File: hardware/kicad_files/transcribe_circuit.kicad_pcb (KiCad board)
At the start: 2 copper layers, 100 x 45 mm, 25 parts, among them J1 europower, J2 RS232_SERIAL, J3 RS232_DSUB, J4 MIDI_IN_TRS, J5 MIDI_IN_DIN, J6 MIDI_OUT_TRS, J7 MIDI_OUT_DIN, J8 Conn_01x06, U1 ProMicro, U2 MAX232, U3 6N137, U4 4069, U5 usbHostMini, U6 L78L33_TO92

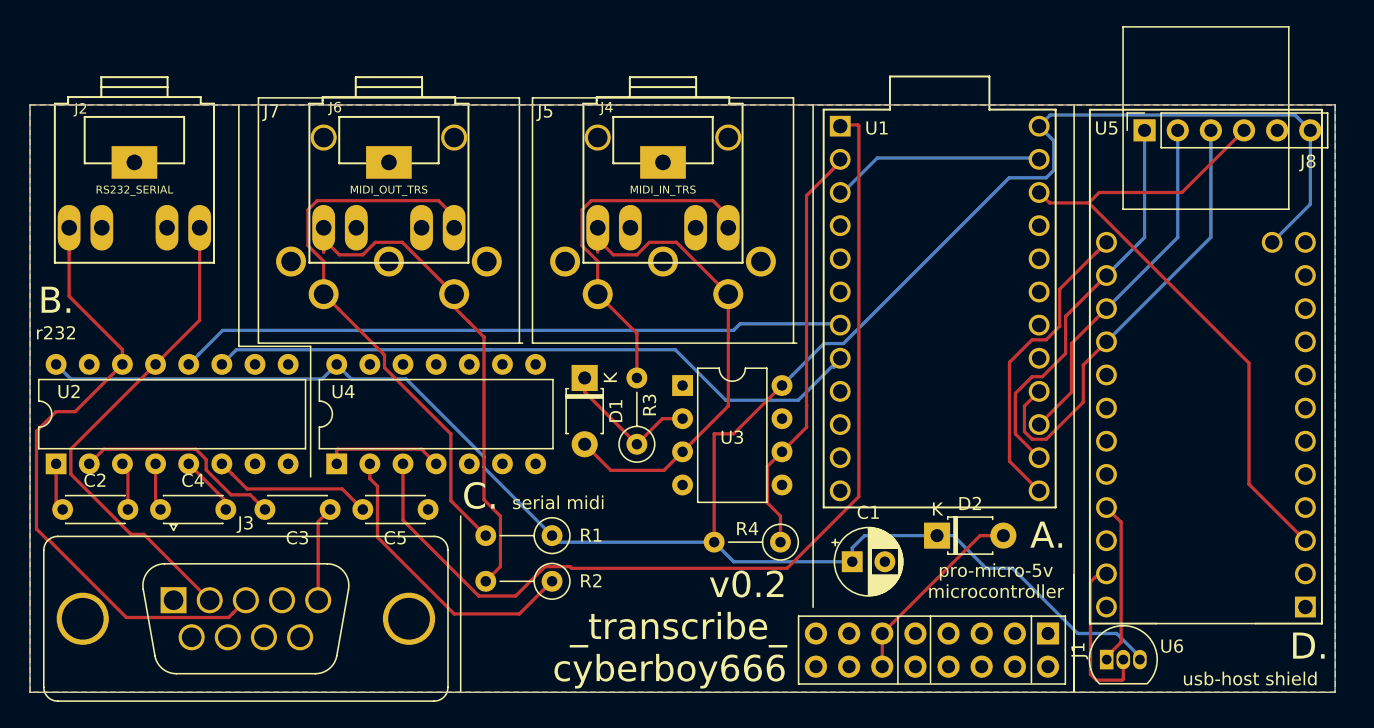
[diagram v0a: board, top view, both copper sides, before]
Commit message: refactored the code and updated circuit
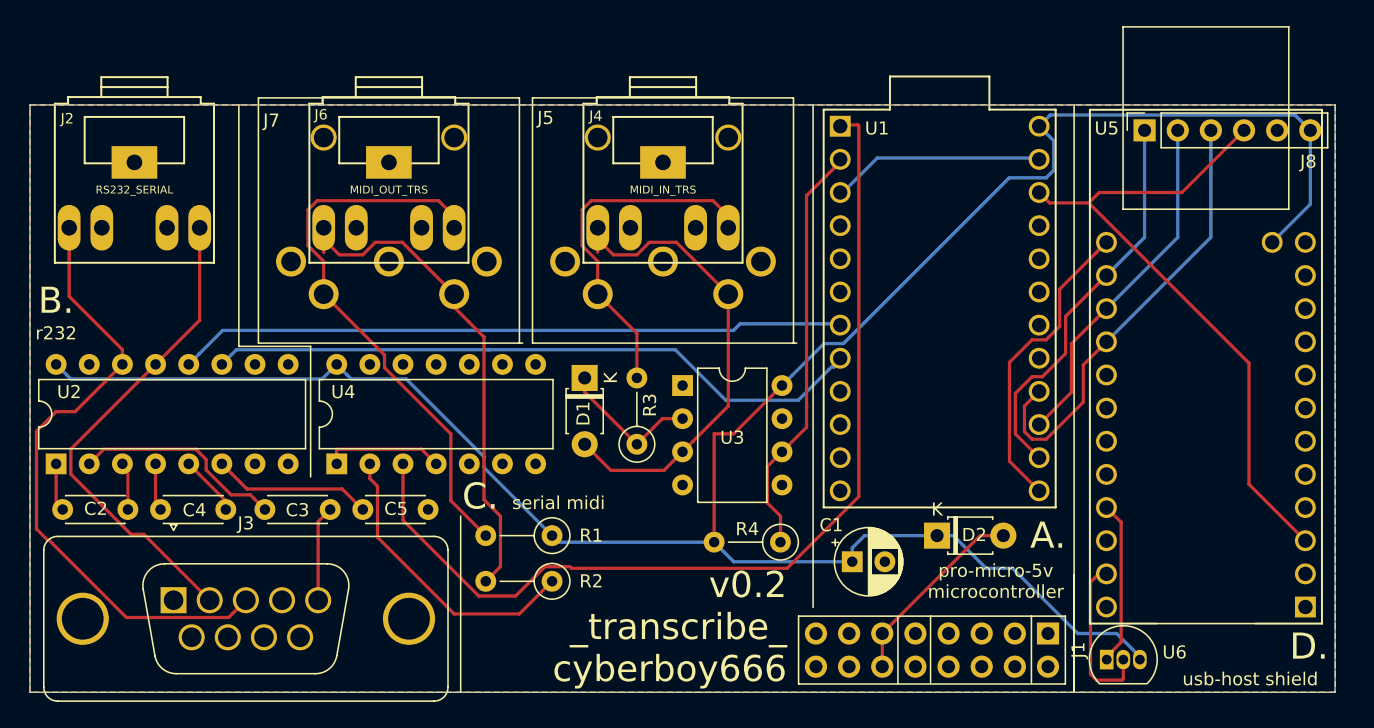
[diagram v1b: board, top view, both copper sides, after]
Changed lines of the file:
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@@
     (pcbplotparams
       (layerselection 0x010fc_ffffffff)
-      (usegerberextensions false)
+      (usegerberextensions true)
       (usegerberattributes false)
       (usegerberadvancedattributes false)
@@
       (drillshape 0)
       (scaleselection 1)
-      (outputdirectory "../transcribe_0.2/"))
+      (outputdirectory "../transcribe_0.2b/"))
   )
   (net 0 "")
@@
     (descr "Diode, T-1 series, Axial, Horizontal, pin pitch=5.08mm, , length*diameter=3.2*2.6mm^2, , http://www.diodes.com/_files/packages/T-1.pdf")
     (tags "Diode T-1 series Axial Horizontal pin pitch 5.08mm  length 3.2mm diameter 2.6mm")
-    (fp_text reference D1 (at 2.54 -2.42 90) (layer F.SilkS)
+    (fp_text reference D1 (at 2.73 0.1 90) (layer F.SilkS)
       (effects (font (size 1 1) (thickness 0.15)))
     )
@@
     (descr "SDS-50J, standard DIN connector, 5 pins, midi")
     (tags "SDS-50J DIN 5-pins connector midi")
-    (fp_text reference J7 (at -1.5 -11.5) (layer F.SilkS)
+    (fp_text reference J7 (at -1.5 -10.8) (layer F.SilkS)
       (effects (font (size 1 1) (thickness 0.15)))
     )
@@
   (module lib_fp:Tayda_3.5mm_stereo_TRS_jack_A-853 (layer F.Cu)
     (at -241.5 -784)
-    (fp_text reference J4 (at -4.3 -5.8) (layer F.SilkS)
+    (fp_text reference J4 (at -5.15 -5.15) (layer F.SilkS)
       (effects (font (size 0.8 0.8) (thickness 0.15)))
     )
@@
     (descr "TO-92 leads in-line, narrow, oval pads, drill 0.75mm (see NXP sot054_po.pdf)")
     (tags "to-92 sc-43 sc-43a sot54 PA33 transistor")
-    (fp_text reference U6 (at 5 -1) (layer F.SilkS)
+    (fp_text reference U6 (at 5.2 -0.55) (layer F.SilkS)
       (effects (font (size 1 1) (thickness 0.15)))
     )
@@
       (effects (font (size 1 1) (thickness 0.15)))
     )
-    (fp_text user %R (at 1.27 -3.56) (layer F.Fab)
+    (fp_text user %R (at 5.15 -0.6) (layer F.Fab)
       (effects (font (size 1 1) (thickness 0.15)))
     )
@@
     (descr "CP, Radial series, Radial, pin pitch=2.50mm, , diameter=5mm, Electrolytic Capacitor")
     (tags "CP Radial series Radial pin pitch 2.50mm  diameter 5mm Electrolytic Capacitor")
-    (fp_text reference C1 (at 1.25 -3.75) (layer F.SilkS)
+    (fp_text reference C1 (at -1.6 -2.8) (layer F.SilkS)
       (effects (font (size 1 1) (thickness 0.15)))
     )
@@
     (descr "C, Disc series, Radial, pin pitch=5.00mm, , diameter*width=4.3*1.9mm^2, Capacitor, http://www.vishay.com/docs/45233/krseries.pdf")
     (tags "C Disc series Radial pin pitch 5.00mm  diameter 4.3mm width 1.9mm Capacitor")
-    (fp_text reference C2 (at 2.5 -2.2) (layer F.SilkS)
+    (fp_text reference C2 (at 2.55 -0.05) (layer F.SilkS)
       (effects (font (size 1 1) (thickness 0.15)))
     )
@@
     (descr "C, Disc series, Radial, pin pitch=5.00mm, , diameter*width=4.3*1.9mm^2, Capacitor, http://www.vishay.com/docs/45233/krseries.pdf")
     (tags "C Disc series Radial pin pitch 5.00mm  diameter 4.3mm width 1.9mm Capacitor")
-    (fp_text reference C3 (at 2.5 -2.2) (layer F.SilkS)
+    (fp_text reference C3 (at 2.5 -0.05) (layer F.SilkS)
       (effects (font (size 1 1) (thickness 0.15)))
     )
@@
     (descr "C, Disc series, Radial, pin pitch=5.00mm, , diameter*width=4.3*1.9mm^2, Capacitor, http://www.vishay.com/docs/45233/krseries.pdf")
     (tags "C Disc series Radial pin pitch 5.00mm  diameter 4.3mm width 1.9mm Capacitor")
-    (fp_text reference C4 (at 2.5 -2.2) (layer F.SilkS)
+    (fp_text reference C4 (at 2.6 0.05) (layer F.SilkS)
       (effects (font (size 1 1) (thickness 0.15)))
     )
@@
     (descr "C, Disc series, Radial, pin pitch=5.00mm, , diameter*width=4.3*1.9mm^2, Capacitor, http://www.vishay.com/docs/45233/krseries.pdf")
     (tags "C Disc series Radial pin pitch 5.00mm  diameter 4.3mm width 1.9mm Capacitor")
-    (fp_text reference C5 (at 2.5 -2.2) (layer F.SilkS)
+    (fp_text reference C5 (at 2.45 0.05) (layer F.SilkS)
       (effects (font (size 1 1) (thickness 0.15)))
     )
@@
     (descr "Diode, T-1 series, Axial, Horizontal, pin pitch=5.08mm, , length*diameter=3.2*2.6mm^2, , http://www.diodes.com/_files/packages/T-1.pdf")
     (tags "Diode T-1 series Axial Horizontal pin pitch 5.08mm  length 3.2mm diameter 2.6mm")
-    (fp_text reference D2 (at 2.54 -2.42) (layer F.SilkS)
+    (fp_text reference D2 (at 2.85 -0.05) (layer F.SilkS)
       (effects (font (size 1 1) (thickness 0.15)))
     )
@@
   (module lib_fp:Tayda_3.5mm_stereo_TRS_jack_A-853 (layer F.Cu)
     (at -282 -784)
-    (fp_text reference J2 (at -4.1 -5.7) (layer F.SilkS)
+    (fp_text reference J2 (at -5.15 -4.95) (layer F.SilkS)
       (effects (font (size 0.8 0.8) (thickness 0.15)))
     )
@@
     (descr "SDS-50J, standard DIN connector, 5 pins, midi")
     (tags "SDS-50J DIN 5-pins connector midi")
-    (fp_text reference J5 (at -1.5 -11.5) (layer F.SilkS)
+    (fp_text reference J5 (at -1.5 -11) (layer F.SilkS)
       (effects (font (size 1 1) (thickness 0.15)))
     )
@@
   (module lib_fp:Tayda_3.5mm_stereo_TRS_jack_A-853 (layer F.Cu)
     (at -262.5 -784)
-    (fp_text reference J6 (at -4.1 -5.8) (layer F.SilkS)
+    (fp_text reference J6 (at -5.2 -5.25) (layer F.SilkS)
       (effects (font (size 0.8 0.8) (thickness 0.15)))
     )
